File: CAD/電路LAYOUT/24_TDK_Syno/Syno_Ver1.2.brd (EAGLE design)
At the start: 55.9 x 65.7 mm, 13 parts, among them IC1 REG1117

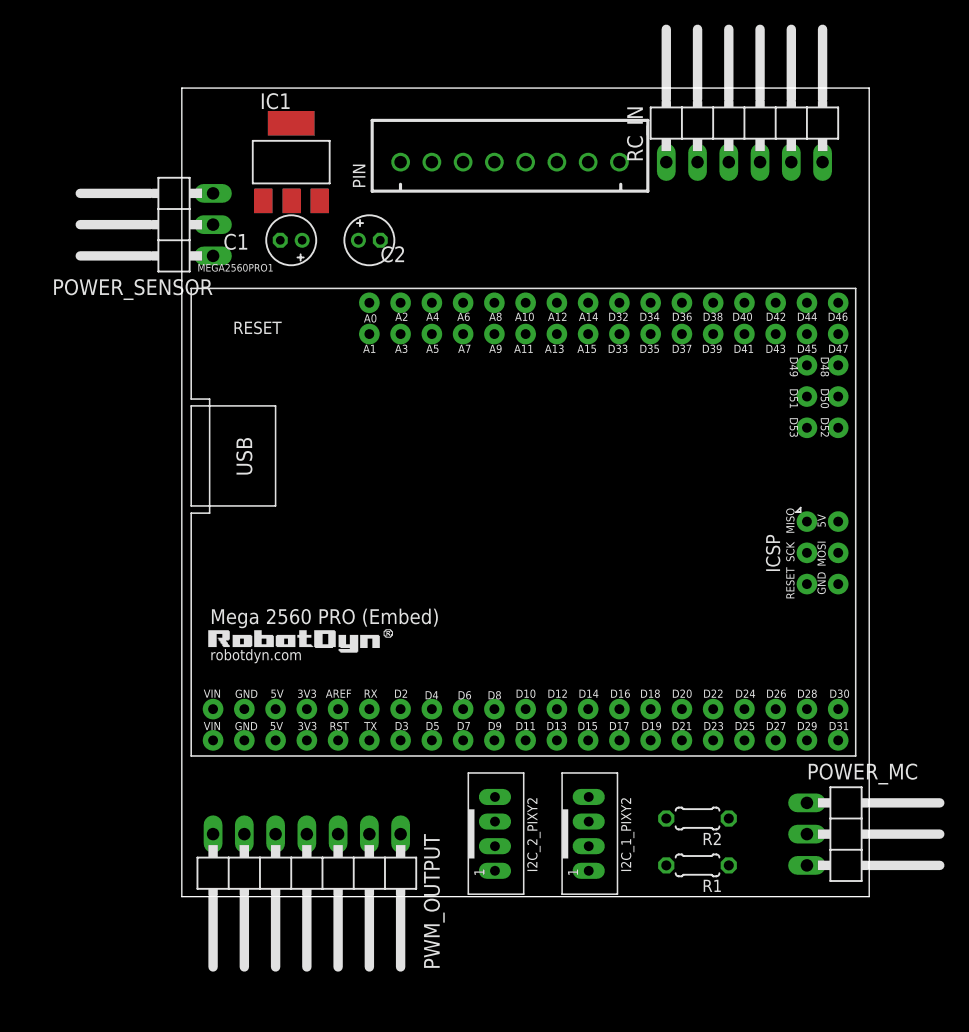
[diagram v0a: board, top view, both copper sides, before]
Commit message: daily update
整理檔案與更新電路Layout(1.0~1.2)
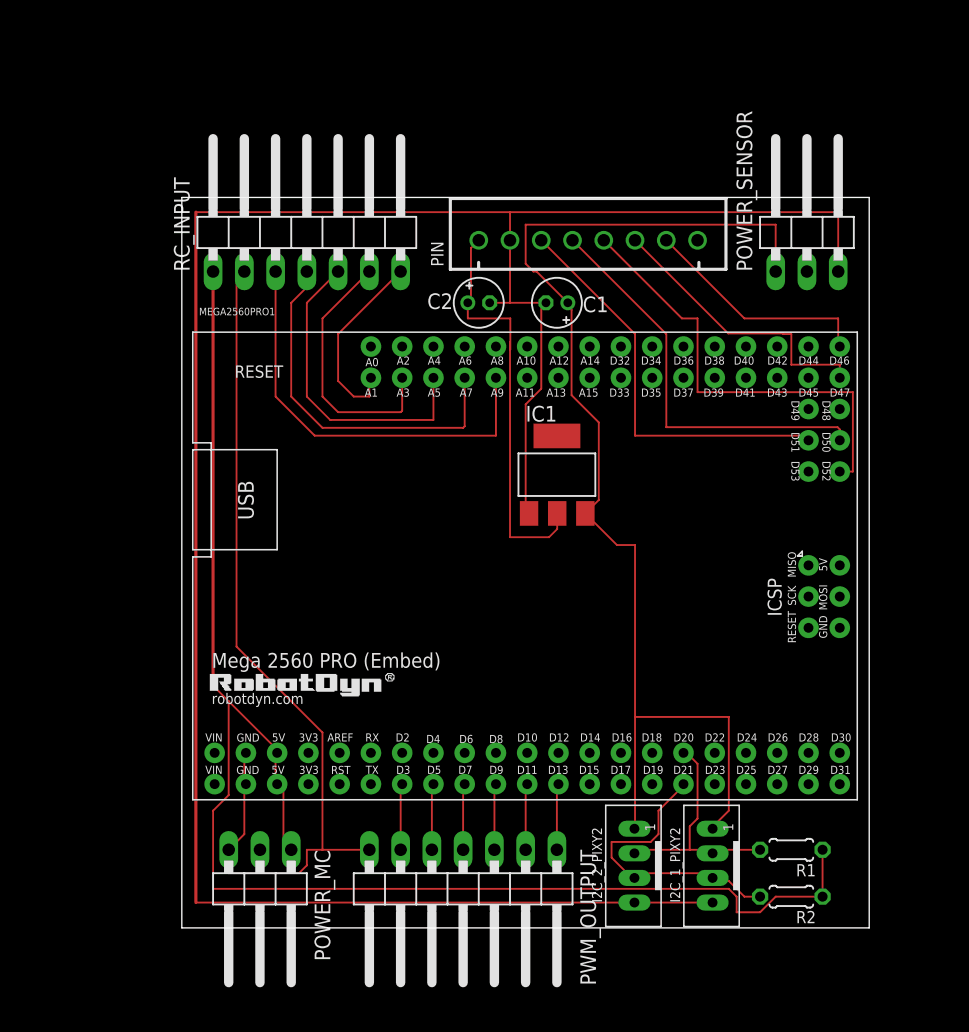
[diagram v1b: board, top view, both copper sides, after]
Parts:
- removed RC_IN: (no value), pinhead:1X06/90
- added RC_INPUT: (no value), pinhead:1X07/90
- moved POWER_SENSOR 52.1 mm to (50.8, 54.6), turned to 0 degrees
- moved POWER_MC 48.5 mm to (6.35, 0.00), turned to 180 degrees
- moved IC1 33.3 mm to (30.5, 34.3)
- moved C1 22.2 mm to (30.5, 48.3)
- moved PWM_OUTPUT 12.8 mm to (22.9, 0.00)
- moved I2C_2_PIXY2 11.7 mm to (36.8, 2.54), turned to 90 degrees
- moved I2C_1_PIXY2 10.5 mm to (43.2, 2.54), turned to 90 degrees
- moved C2 10.2 mm to (24.1, 48.3)
- moved R2 9.92 mm to (49.5, 0.00)
- moved PIN 8.98 mm to (33.0, 53.3)
- moved R1 7.73 mm to (49.5, 3.81)
- moved MEGA2560PRO1 3.56 mm to (35.7, 28.2)
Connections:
- removed net N$18: MEGA2560PRO1.D40, RC_IN.5
- removed net N$19: MEGA2560PRO1.GND@2, RC_IN.6
- net 5V: now also MEGA2560PRO1.5V@1, MEGA2560PRO1.5V@2, RC_INPUT.1
- net GND: now also MEGA2560PRO1.GND@1, MEGA2560PRO1.GND@2, PWM_OUTPUT.7, RC_INPUT.2
- net N$13: now also MEGA2560PRO1.A9, RC_INPUT.3; no longer MEGA2560PRO1.GND@1, PWM_OUTPUT.7
- net N$14: now also MEGA2560PRO1.A7, RC_INPUT.4; no longer MEGA2560PRO1.D32, RC_IN.1
- net N$15: now also MEGA2560PRO1.A5, RC_INPUT.5; no longer MEGA2560PRO1.D34, RC_IN.2
- net N$16: now also MEGA2560PRO1.A3, RC_INPUT.6; no longer MEGA2560PRO1.D36, RC_IN.3
- net N$17: now also MEGA2560PRO1.A1, RC_INPUT.7; no longer MEGA2560PRO1.D38, RC_IN.4
- net N$5: now also MEGA2560PRO1.D47; no longer MEGA2560PRO1.D30
- net N$6: now also MEGA2560PRO1.D46; no longer MEGA2560PRO1.D31
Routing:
- net GND_S: track 0.00 -> 184.8 mm
- net 5V: track 0.00 -> 120.9 mm
- net 5V_S: track 0.00 -> 96.4 mm
- net GND: track 0.00 -> 73.8 mm
- net N$4: track 0.00 -> 36.4 mm
- net N$2: track 0.00 -> 34.1 mm
- net N$13: track 0.00 -> 34.1 mm
- net N$3: track 0.00 -> 33.8 mm
- net N$1: track 0.00 -> 33.4 mm
- net N$14: track 0.00 -> 29.8 mm
- net N$15: track 0.00 -> 25.7 mm
- net SCL: track 0.00 -> 24.2 mm
- net N$5: track 0.00 -> 23.3 mm
- net N$16: track 0.00 -> 21.5 mm
- net SDA: track 0.00 -> 19.5 mm
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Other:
- board size 55.9 x 65.7 mm -> 55.9 x 59.4 mm
